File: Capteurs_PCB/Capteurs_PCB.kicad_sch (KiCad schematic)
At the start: 1 part, among them J1 Raspberry_Pi_2_3

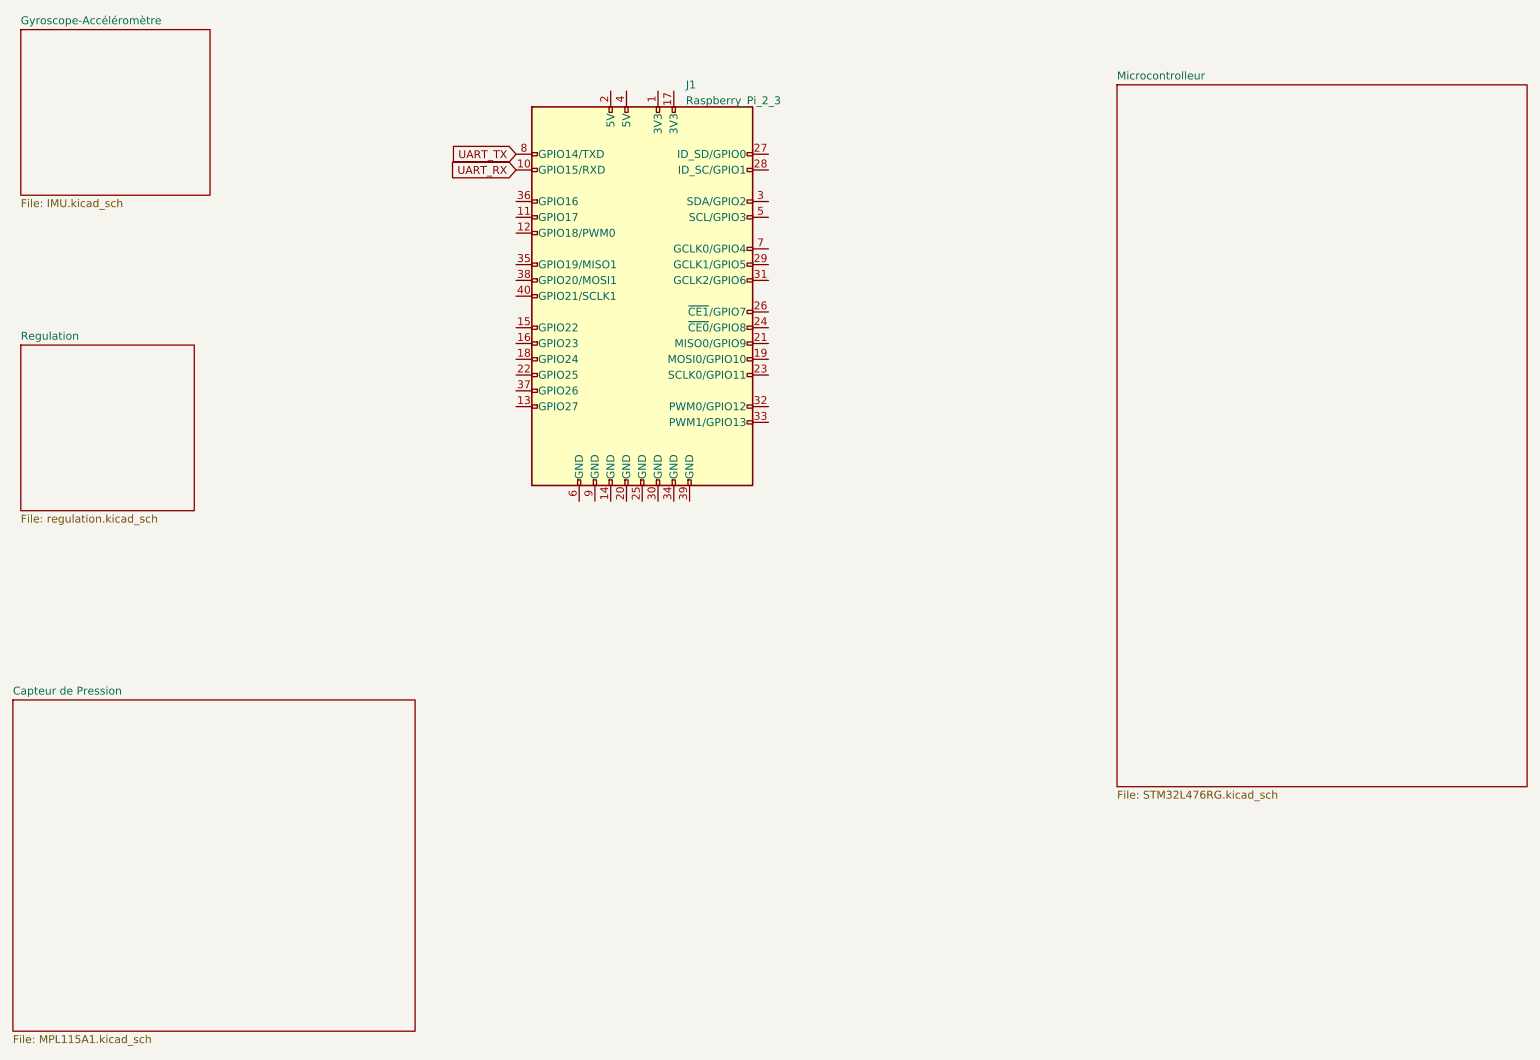
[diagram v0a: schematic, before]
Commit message: pcb update
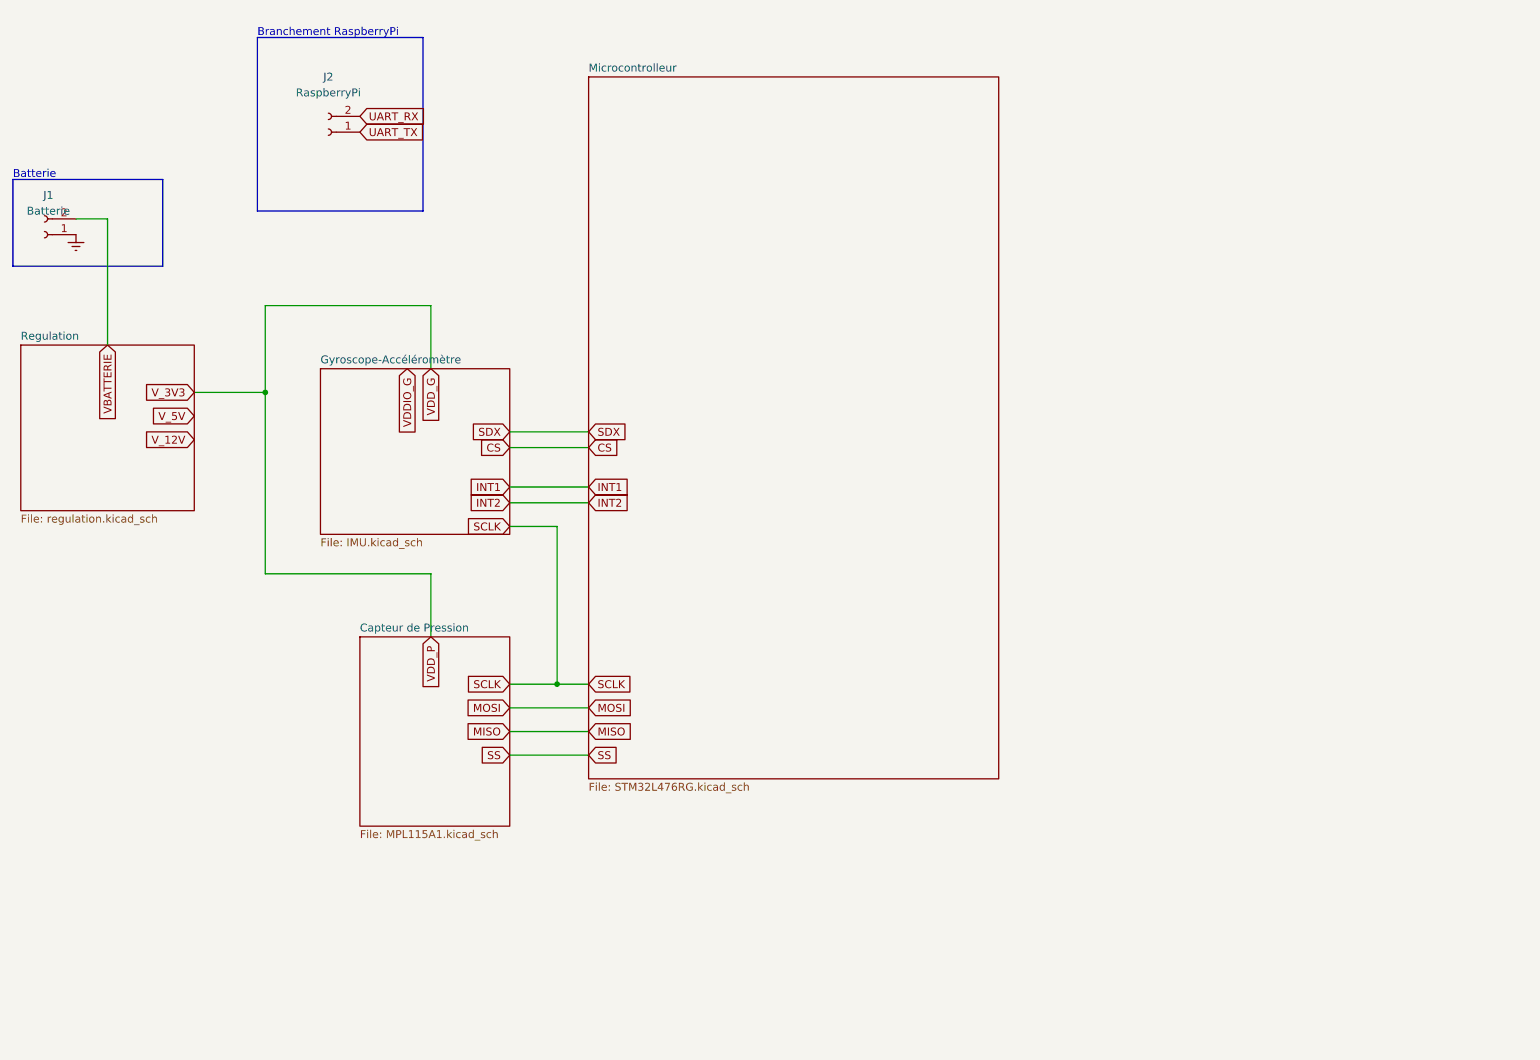
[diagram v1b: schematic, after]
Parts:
- removed J1: Raspberry_Pi_2_3, symbol Connector:Raspberry_Pi_2_3
- added J1: Batterie, symbol Connector:Conn_01x02_Socket
- added J2: RaspberryPi, symbol Connector:Conn_01x02_Socket
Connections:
- net UART_RX: now also J2.2 (Pin_2)
- net UART_TX: now also J2.1 (Pin_1)
- new net Earth: J1.1 (Pin_1)
- new net VBATTERIE: J1.2 (Pin_2)
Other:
- note added: "Batterie"
- note added: "Branchement RaspberryPi"
